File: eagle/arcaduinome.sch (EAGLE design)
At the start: 0 parts

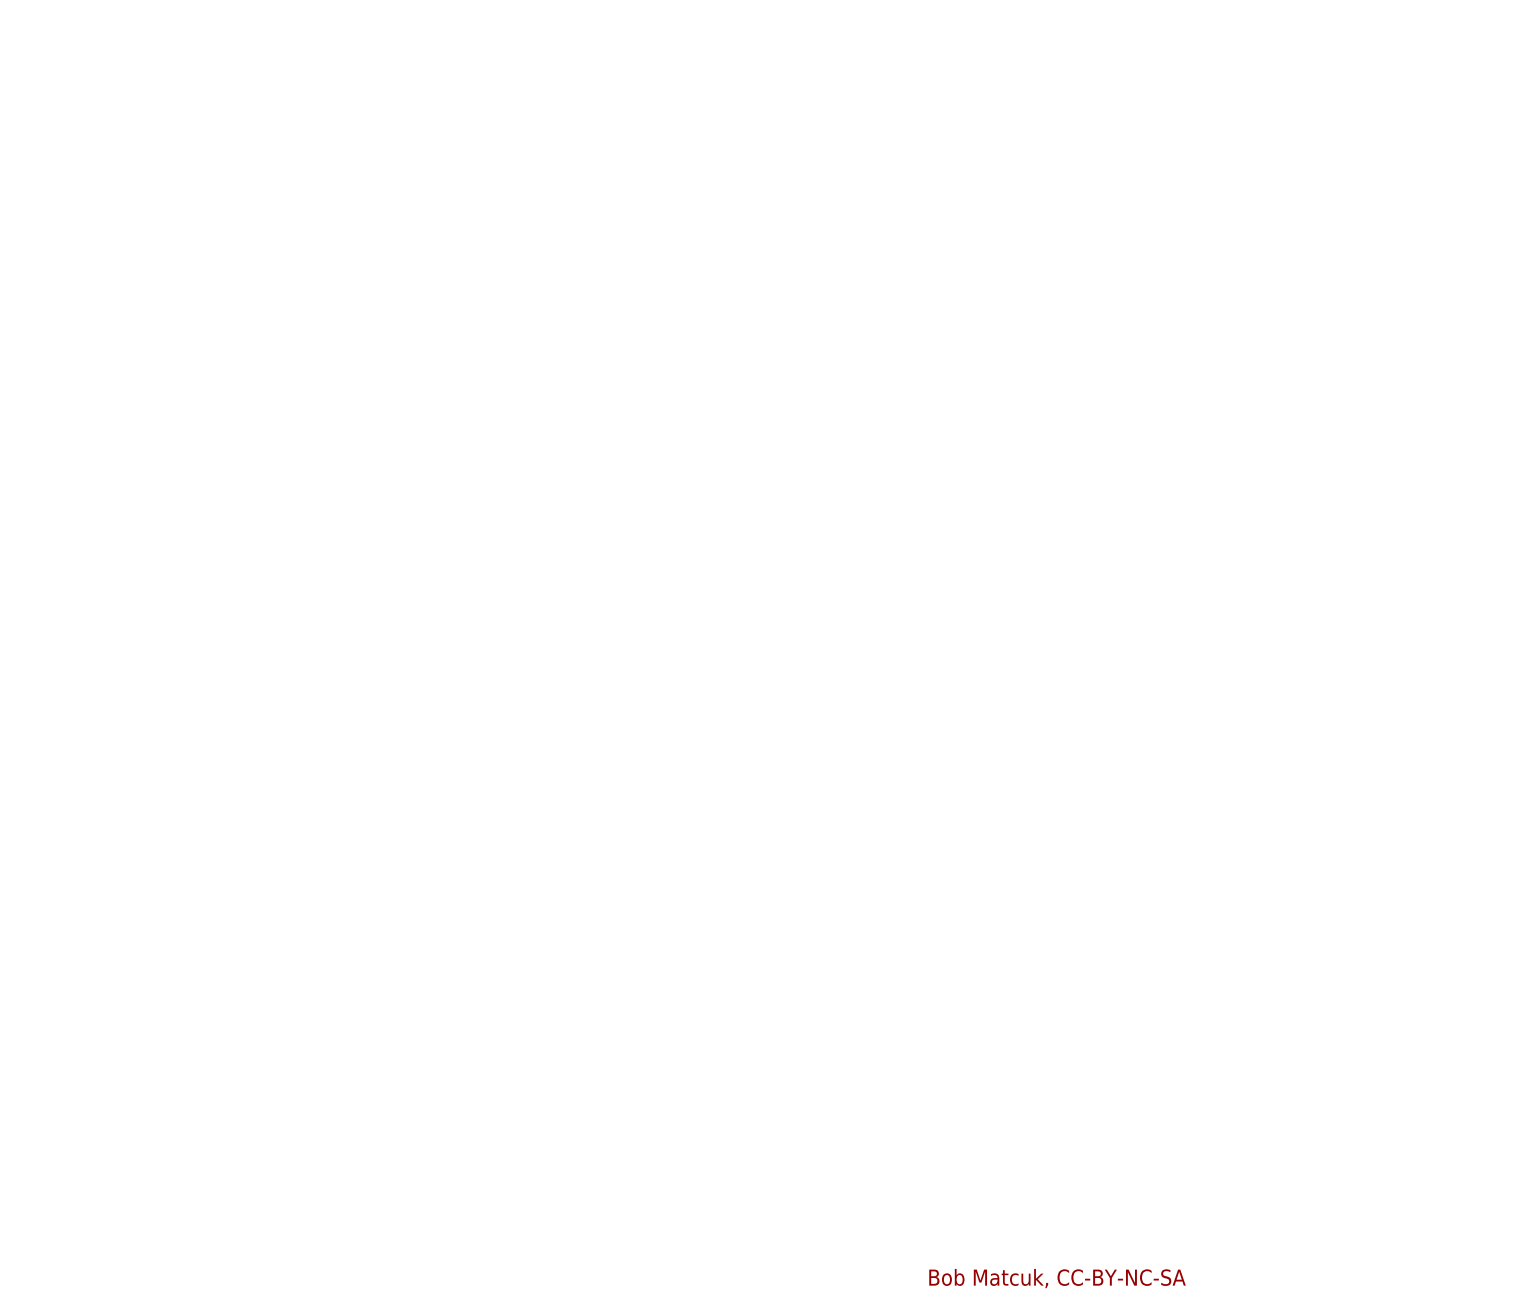
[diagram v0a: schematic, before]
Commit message: made schematic
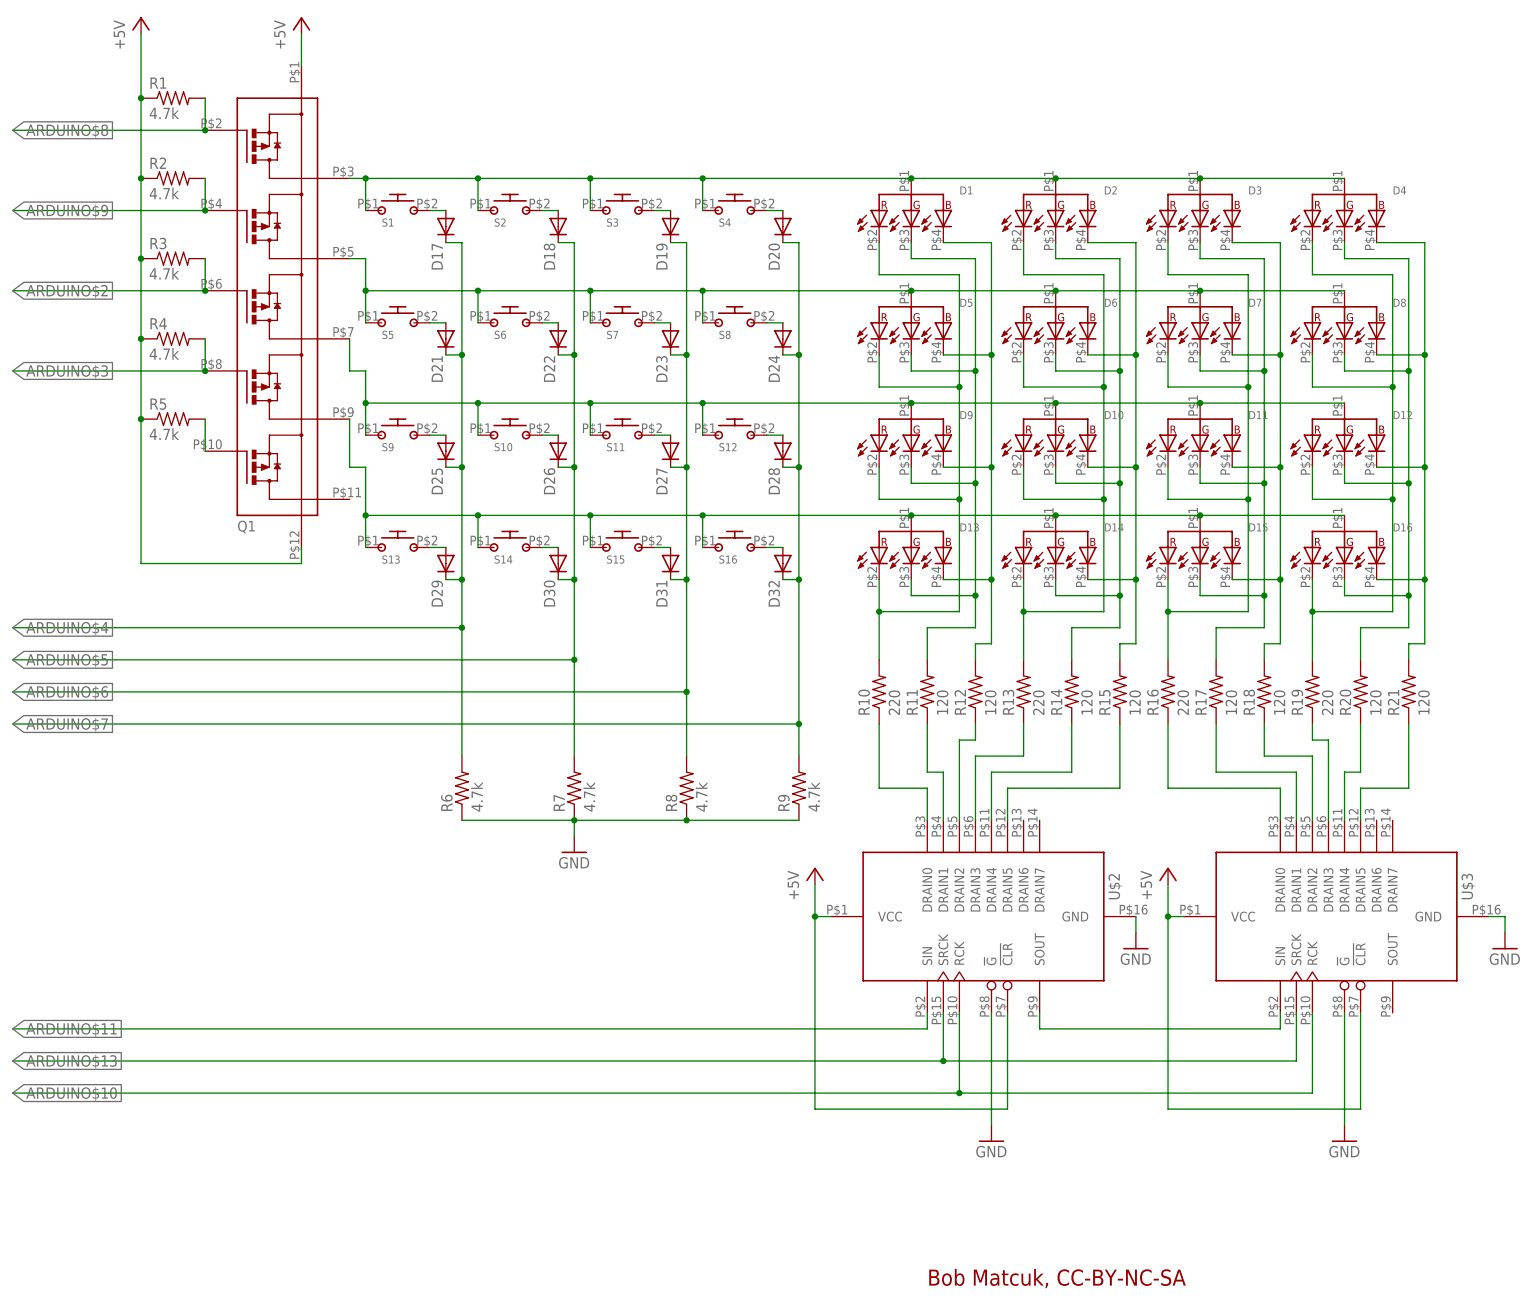
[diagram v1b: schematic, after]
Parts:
- added D1, D10, D11, D12, D13, D14, D15, D16, D2, D3, D4, D5, D6, D7, D8, D9: FD-5WSRGB-A, arcaduinome:FD-5WSRGB-A
- added D17, D18, D19, D20, D21, D22, D23, D24, D25, D26, D27, D28, D29, D30, D31, D32: 1N4148DO35-7, diode:1N4148DO35-7
- added Q1: SLA5086, arcaduinome:SLA5086
- added R1, R2, R3, R4, R5, R6, R7, R8, R9: 4.7k, resistor:R-US_0207/10
- added R10, R13, R16, R19: 220, resistor:R-US_0207/7
- added R11, R12, R14, R15, R17, R18, R20, R21: 120, resistor:R-US_0204/5
- added S1, S10, S11, S12, S13, S14, S15, S16, S2, S3, S4, S5, S6, S7, S8, S9: SANWA_OBSC_24_CW, arcaduinome:SANWA_OBSC_24_CW
- added U$2, U$3: (no value), arcaduinome:STPIC6D595
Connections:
- new net +5V: Q1.S@1, Q1.S@2, R1.1, R2.1, R3.1, R4.1, R5.1, U$2.!CLR, U$2.VCC, U$3.!CLR, U$3.VCC
- new net ARDUINO$10: U$2.RCK, U$3.RCK
- new net ARDUINO$11: U$2.SIN
- new net ARDUINO$13: U$2.SRCK, U$3.SRCK
- new net ARDUINO$2: Q1.G$3, R3.2
- new net ARDUINO$3: Q1.G$4, R4.2
- new net ARDUINO$4: D17.C, D21.C, D25.C, D29.C, R6.2
- new net ARDUINO$5: D18.C, D22.C, D26.C, D30.C, R7.2
- new net ARDUINO$6: D19.C, D23.C, D27.C, D31.C, R8.2
- new net ARDUINO$7: D20.C, D24.C, D28.C, D32.C, R9.2
- new net ARDUINO$8: Q1.G$1, R1.2
- new net ARDUINO$9: Q1.G$2, R2.2
- new net GND: R6.1, R7.1, R8.1, R9.1, U$2.!G, U$2.GND, U$3.!G, U$3.GND
- new net N$1: D1.ANODE, D2.ANODE, D3.ANODE, D4.ANODE, Q1.D$1, S1.P$1, S2.P$1, S3.P$1, S4.P$1
- new net N$10: D23.A, S7.P$2
- new net N$11: D24.A, S8.P$2
- new net N$16: D10.ANODE, D11.ANODE, D12.ANODE, D9.ANODE, Q1.D$3, S10.P$1, S11.P$1, S12.P$1, S9.P$1
- new net N$17: D25.A, S9.P$2
- new net N$18: D26.A, S10.P$2
- new net N$19: D27.A, S11.P$2
- new net N$2: D17.A, S1.P$2
- new net N$20: D28.A, S12.P$2
- new net N$21: D13.ANODE, D14.ANODE, D15.ANODE, D16.ANODE, Q1.D$4, S13.P$1, S14.P$1, S15.P$1, S16.P$1
- new net N$22: D29.A, S13.P$2
- new net N$23: D30.A, S14.P$2
- new net N$24: D31.A, S15.P$2
- new net N$25: D32.A, S16.P$2
- new net N$26: D1.R, D13.R, D5.R, D9.R, R10.2
- new net N$27: D1.G, D13.G, D5.G, D9.G, R11.2
- new net N$28: D1.B, D13.B, D5.B, D9.B, R12.2
- new net N$29: D10.R, D14.R, D2.R, D6.R, R13.2
- new net N$3: D18.A, S2.P$2
- new net N$30: D10.G, D14.G, D2.G, D6.G, R14.2
- new net N$31: D10.B, D14.B, D2.B, D6.B, R15.2
- new net N$32: D11.R, D15.R, D3.R, D7.R, R16.2
- new net N$33: D11.G, D15.G, D3.G, D7.G, R17.2
- new net N$34: D11.B, D15.B, D3.B, D7.B, R18.2
- new net N$35: D12.R, D16.R, D4.R, D8.R, R19.2
- new net N$36: D12.G, D16.G, D4.G, D8.G, R20.2
- new net N$37: D12.B, D16.B, D4.B, D8.B, R21.2
- new net N$38: R10.1, U$2.DRAIN0
- new net N$39: R11.1, U$2.DRAIN1
- new net N$4: D19.A, S3.P$2
- new net N$40: R15.1, U$2.DRAIN5
- new net N$41: R14.1, U$2.DRAIN4
- new net N$42: R13.1, U$2.DRAIN3
- new net N$43: R12.1, U$2.DRAIN2
- new net N$44: R21.1, U$3.DRAIN5
- new net N$45: R20.1, U$3.DRAIN4
- new net N$46: R16.1, U$3.DRAIN0
- new net N$47: R17.1, U$3.DRAIN1
- new net N$48: R18.1, U$3.DRAIN2
- new net N$49: R19.1, U$3.DRAIN3
- new net N$5: Q1.G$5, R5.2
- new net N$54: U$2.SOUT, U$3.SIN
- new net N$6: D20.A, S4.P$2
- new net N$7: D5.ANODE, D6.ANODE, D7.ANODE, D8.ANODE, Q1.D$2, S5.P$1, S6.P$1, S7.P$1, S8.P$1
- new net N$8: D21.A, S5.P$2
- new net N$9: D22.A, S6.P$2
